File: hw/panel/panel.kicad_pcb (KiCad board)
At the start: 4 copper layers, 158 x 89 mm, 296 parts, among them J1 Input, J1 USB_OTG, J2 BATT, J2 Output, J201 Modem, J202 SIM_Card, J203 Motor, J204 Micro_SD_Card, J205 Prog, J206 Expansion, J207 Camera, J3 +5V, J301 iMX8, J305 Micro_SD_Card, J4 SJ-3571N, J401 Touch, J402 Display, J5 SPEAKER, SW1 RESET, SW2 WAKE, SW201 BOOT, SW202 PERST, U1 BQ25895, U1 SN65LVDS822, U10 74HC595, U11 ICS-43434, U12 MAX98357A, U13 MAX98357A, U14 SN74LVC1G04DCK, U15 SN74LVC1G3157DCK, U16 SN74LVC2G07DCK, U2 SN74LVC00ARGY, U2 TPS62293, U201 ESP32-WROOM, U202 SN74CBTLV3125RGY, U203 TXB0104RGY, U204 TXB0104RGY, U205 DRV2605LDGS, U206 LSM9DS1, U207 FT230XQ, U208 TMUX154ERSW, U3 TPS630250, U4 FE310-G002, U401 FAN5333BSX, U402 SN74LVC3G06DCU, U403 BT817Q, U404 IS25LP128-JKLE, U405 DS90C185, U406 TS3DV520ERUA, U407 TXS0104ERGY, U408 TXS0104ERGY, U409 SN74LVC2G06DCK, U5 IS25LP128-JKLE, U6 TMUX1574RSV, U7 74HC00, U8 74HC00, U9 74HC595, X1 SiT1533, Y1 16MHz, Y401 12MHz

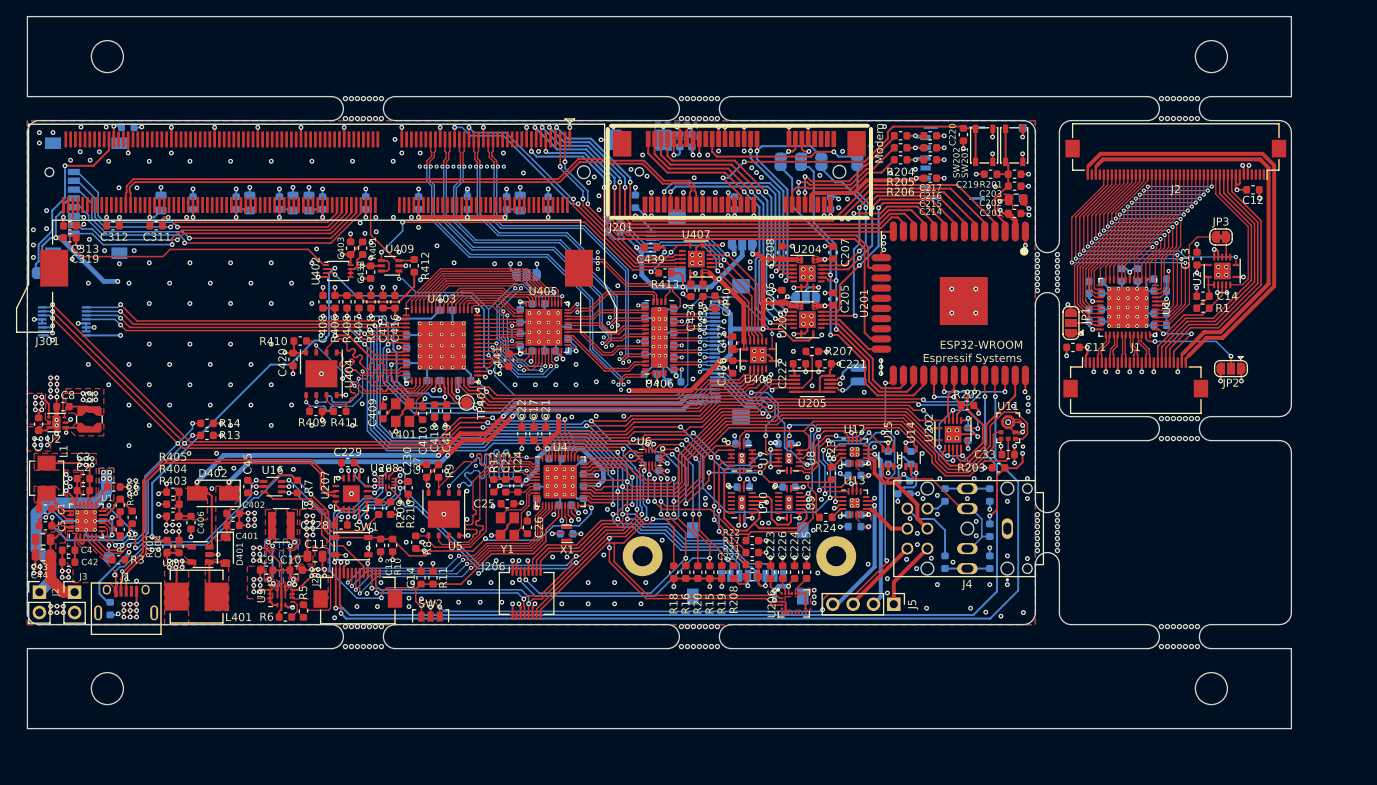
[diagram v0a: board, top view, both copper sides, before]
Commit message: temp commit for merge
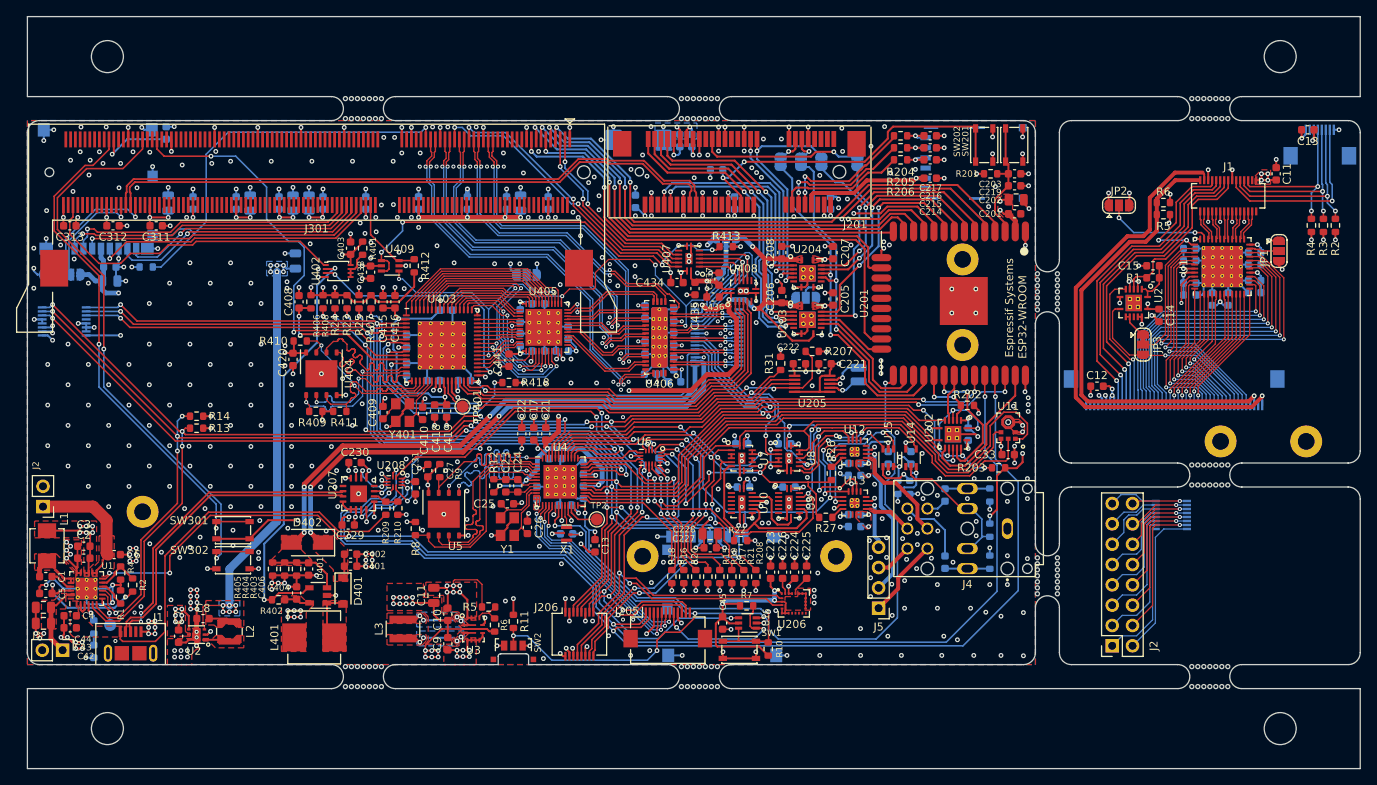
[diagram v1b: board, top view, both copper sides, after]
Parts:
- removed the C1 at (189.5, 86.6)
- removed the C1 at (58.2, 111.5)
- removed the C11 at (186.7, 91.3)
- removed the C11 at (92.0, 117.5)
- removed C439, C440: 0.1uF, Capacitor_SMD:C_0603_1608Metric
- removed the J1 at (194.6, 95.1)
- removed the J1 at (68.3, 123.4)
- removed the J2 at (199.6, 67.9)
- removed the J2 at (57.5, 122.0)
- removed the J3 at (61.9, 122.0)
- removed J305: Micro_SD_Card, footprints:microSD
- removed the R2 at (69.1, 112.6)
- removed the R3 at (67.4, 117.9)
- removed the R4 at (67.6, 111.1)
- removed R414, R415: R, Resistor_SMD:R_0603_1608Metric
- removed the R5 at (90.5, 124.3)
- removed the R6 at (88.2, 125.0)
- removed the REF** at (183.5, 114.5)
- removed the REF** at (183.5, 82.0)
- removed the REF** at (98.0, 127.5)
- removed the REF** at (140.0, 127.5)
- removed the REF** at (200.0, 127.5)
- removed the REF** at (200.0, 101.5)
- removed the REF** at (200.0, 61.5)
- removed the U2 at (205.3, 81.8)
- removed the U2 at (59.6, 100.8)
- added C1: 47nF, Capacitor_SMD:C_0603_1608Metric, F.Cu at (58.3, 120.0)
- added C1: 0.1uF, Capacitor_SMD:C_0603_1608Metric, B.Cu at (209.4, 81.0)
- added C11: 47uF, Capacitor_SMD:C_0805_2012Metric, F.Cu at (106.8, 122.3)
- added C11: 10uF, Capacitor_SMD:C_0603_1608Metric, F.Cu at (212.1, 69.7)
- added C13: 0.1uF, Capacitor_SMD:C_0603_1608Metric, F.Cu at (216.1, 64.2)
- added C228: 22uF, Capacitor_SMD:C_0805_2012Metric, F.Cu at (141.3, 114.7)
- added C320: 22uF, Capacitor_SMD:C_0805_2012Metric, B.Cu at (66.3, 83.0)
- added J1: USB_OTG, footprints:GCT_MicroUSB-USB3080, F.Cu at (68.9, 126.9)
- added J1: Input, Connector_Molex:Molex_SlimStack_55560-0301_2x15_P0.50mm_Vertical, F.Cu at (206.1, 72.4)
- added J1: In, Connector_Molex:Molex_SlimStack_55560-0161_2x08_P0.50mm_Vertical, B.Cu at (199.0, 112.3)
- added J2: BATT, Connector_PinHeader_2.54mm:PinHeader_1x02_P2.54mm_Vertical, F.Cu at (58.0, 111.2)
- added J2: Display, Connector_FFC-FPC:Hirose_FH12-45S-0.5SH_1x45-1MP_P0.50mm_Horizontal, B.Cu at (199.3, 96.7)
- added J2: Out, Connector_PinHeader_2.54mm:PinHeader_2x08_P2.54mm_Vertical, F.Cu at (191.6, 128.7)
- added J3: +5V, Connector_PinHeader_2.54mm:PinHeader_1x02_P2.54mm_Vertical, F.Cu at (60.4, 129.2)
- added J3: Touch, Connector_FFC-FPC:Hirose_FH12-8S-0.5SH_1x08-1MP_P0.50mm_Horizontal, B.Cu at (217.6, 66.0)
- added J302: Micro_SD_Card_Det, footprints:Molex_MicroSD-5027740891, B.Cu at (70.8, 63.3)
- added J303: Spacer, footprints:Spacer, F.Cu at (70.4, 111.9)
- added J4: Spacer, footprints:Spacer, F.Cu at (215.8, 103.1)
- added J403: Spacer, footprints:Spacer, B.Cu at (172.9, 91.0)
- added J5: Spacer, footprints:Spacer, F.Cu at (205.2, 103.1)
- added JP302: USB_ID, Jumper:SolderJumper-2_P1.3mm_Open_RoundedPad1.0x1.5mm, B.Cu at (58.6, 82.2)
- added R2: 10K, Resistor_SMD:R_0603_1608Metric, F.Cu at (69.2, 121.0)
- added R2: DNP, Resistor_SMD:R_0603_1608Metric, F.Cu at (219.5, 76.1)
- added R23: 100K, Resistor_SMD:R_0603_1608Metric, F.Cu at (96.0, 85.7)
- added R24: 100K, Resistor_SMD:R_0603_1608Metric, F.Cu at (94.5, 85.7)
- added R25: 100K, Resistor_SMD:R_0603_1608Metric, F.Cu at (97.5, 85.7)
- added R3: 2.2K, Resistor_SMD:R_0603_1608Metric, B.Cu at (64.3, 126.3)
- added R3: DNP, Resistor_SMD:R_0603_1608Metric, F.Cu at (218.0, 76.1)
- added R301: 100K, Resistor_SMD:R_0603_1608Metric, B.Cu at (70.8, 81.3)
- added R31: 100K, Resistor_SMD:R_0603_1608Metric, F.Cu at (150.2, 93.3)
- added R4: 10K, Resistor_SMD:R_0603_1608Metric, F.Cu at (67.7, 119.5)
- added R4: DNP, Resistor_SMD:R_0603_1608Metric, F.Cu at (216.5, 76.1)
- added R5: 560K, Resistor_SMD:R_0603_1608Metric, F.Cu at (113.7, 123.8)
- added R5: DNP, Resistor_SMD:R_0603_1608Metric, F.Cu at (198.0, 74.8)
- added R6: 180K, Resistor_SMD:R_0603_1608Metric, F.Cu at (114.4, 126.0)
- added R6: DNP, Resistor_SMD:R_0603_1608Metric, F.Cu at (198.0, 73.2)
- added REF**: mouse-bite-3mm-slot, panelization:mouse-bite-3mm-slot, F.Cu at (183.5, 119.9)
- added REF**: mouse-bite-3mm-slot, panelization:mouse-bite-3mm-slot, F.Cu at (183.5, 84.4)
- added REF**: mouse-bite-3mm-slot, panelization:mouse-bite-3mm-slot, F.Cu at (98.0, 132.5)
- added REF**: mouse-bite-3mm-slot, panelization:mouse-bite-3mm-slot, F.Cu at (140.0, 132.5)
- added REF**: mouse-bite-3mm-slot, panelization:mouse-bite-3mm-slot, F.Cu at (203.8, 132.5)
- added REF**: mouse-bite-3mm-slot, panelization:mouse-bite-3mm-slot, F.Cu at (203.8, 107.3)
- added REF**: mouse-bite-3mm-slot, panelization:mouse-bite-3mm-slot, F.Cu at (203.8, 61.5)
- added SW301: iMX8_ALT_BOOT, Button_Switch_SMD:SW_SPST_PTS810, F.Cu at (81.7, 114.2)
- added SW302: iMX8_RST, Button_Switch_SMD:SW_SPST_PTS810, F.Cu at (81.7, 118.0)
- added TP2: PMU_OUT0, TestPoint:TestPoint_Pad_D1.5mm, F.Cu at (127.2, 112.8)
- added U2: TPS62293, footprints:TPS62290, F.Cu at (77.2, 127.2)
- added U2: SN74LVC00ARGY, footprints:Texas_S-PVQFN-N14_ThermalVias, F.Cu at (194.3, 85.8)
- C14: value 10nF -> 22uF; footprint Capacitor_SMD:C_0603_1608Metric -> Capacitor_SMD:C_0805_2012Metric; moved to B.Cu
- C219: value 10nF -> 0.1uF
- C220: value 10nF -> 0.1uF; moved to B.Cu
- C319: moved to B.Cu
- J201: footprint footprints:Socket_mPCIe -> footprints:TE_mPCIe-1775862
- J204: value Micro_SD_Card -> Micro_SD_Card_Det; footprint footprints:microSD -> footprints:Molex_MicroSD-5027740891
- J301: footprint footprints:Socket_SODIMM_DDR3_TE_2013289 -> footprints:TE_SODIMMDDR3-2013289
- J401: value Touch -> Display; footprint Connector_FFC-FPC:Hirose_FH12-8S-0.5SH_1x08-1MP_P0.50mm_Horizontal -> Connector_Molex:Molex_SlimStack_54722-0304_2x15_P0.50mm_Vertical
- J402: value Display -> Spacer; footprint Connector_FFC-FPC:Hirose_FH12-26S-0.5SH_1x26-1MP_P0.50mm_Horizontal -> footprints:Spacer
- JP201: value LEVEL EN -> SIMCom_EN
- JP3: footprint Jumper:SolderJumper-2_P1.3mm_Bridged_RoundedPad1.0x1.5mm -> Jumper:SolderJumper-3_P1.3mm_Bridged12_RoundedPad1.0x1.5mm
- JP301: value ALT_BOOT -> USB_VBUS
- L2: footprint footprints:L_Coilcraft_LPS3015 -> footprints:Coilcraft-LPS3015
- L3: footprint footprints:L_Coilcraft_XAL40 -> footprints:Coilcraft-XAL40
- L401: footprint footprints:L_Murata_LQH66SN -> footprints:Murata-LQH66SN
- SW201: value BOOT -> ESP32_RST
- SW202: value PERST -> MODEM_RST
- U10, U9: footprint footprints:74HC595BQ115 -> footprints:DHVQFN-16_2.5x3.5mm_P0.5mm_EP1.0x2.0mm
- U202, U203, U204: footprint Package_DFN_QFN:Texas_S-PVQFN-N14_ThermalVias -> footprints:Texas_S-PVQFN-N14_ThermalVias
- U407, U408: footprint Package_DFN_QFN:Texas_S-PVQFN-N14_ThermalVias -> footprints:DHVQFN-14_2.5x3.0mm_P0.5mm_EP1.0x1.5mm
- U7, U8: footprint footprints:74HC00BQ115 -> footprints:DHVQFN-14_2.5x3.0mm_P0.5mm_EP1.0x1.5mm
- moved C45 61.8 mm to (142.9, 125.8)
- moved U16 61.8 mm to (146.0, 125.8)
- moved R7 58.1 mm to (145.9, 123.7), turned to 0 degrees
- moved SW1 50.2 mm to (145.0, 129.2)
- moved R10 48.7 mm to (148.6, 129.1)
- moved C14 42.6 mm to (89.5, 80.5)
- moved J205 39.1 mm to (136.1, 126.3)
- moved C7 31.8 mm to (74.9, 127.5)
- moved C8 31.8 mm to (78.0, 125.2)
- moved L2 31.8 mm to (81.2, 126.8)
- moved C12 31.4 mm to (189.7, 96.2), turned to 180 degrees
- moved J402 31.3 mm to (172.9, 80.3), turned to 0 degrees
- moved C220 31.2 mm to (142.2, 69.2), turned to 180 degrees
- moved JP1 27.5 mm to (212.4, 79.3), turned to 270 degrees
- moved C13 26.8 mm to (127.0, 116.2)
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- renumbered C13 to C14, C14 to C15, C228 to C229, C229 to C230, C230 to C231, R23 to R26, R24 to R27, R25 to R28, R26 to R29, R27 to R30, R28 to R32, R29 to R33
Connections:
- net Net-(TP401-Pad1) renamed /disp/BT81X_AUDIO
- net Net-(U4-Pad17) renamed /AON_PMU_OUT_1
- C14 pad 1: WAKE -> +1V8
- J204 pad 2: SPI1.SS3 -> GPIO_0
- J204 pad 9: GND -> Net-(J204-Pad9)
- J206 pad 10: UART0.TXD -> TMUX.I2C0.SCL
- J206 pad 11: SPI1.MOSI -> GND
- J206 pad 13: SPI1.MISO -> UART0.TXD
- J206 pad 14: TMUX.I2C0.SDA -> TMUX.GPIO1
- J206 pad 15: SPI1.SCK -> UART0.RXD
- J206 pad 16: TMUX.I2C0.SCL -> TMUX.GPIO0
- J206 pad 5: TMUX.GPIO0 -> SPI1.MOSI
- J206 pad 7: TMUX.GPIO1 -> SPI1.MISO
- J206 pad 8: UART0.RXD -> TMUX.I2C0.SDA
- J206 pad 9: GND -> SPI1.SCK
- J207 pad 1: GPIO_23 -> TMUX.I2C0.SCL
- J207 pad 3: TMUX.I2C0.SCL -> TMUX.I2C0.SDA
- J207 pad 5: TMUX.I2C0.SDA -> SPI1.SS2
- J207 pad 8: BT81X.GPIO0 -> Net-(J207-Pad8)
- J301 pad 165: Net-(J301-Pad165) -> BT81X.GPIO0
- J301 pad 171: Net-(J301-Pad171) -> /exp/RESET
- J301 pad 174: Net-(J301-Pad174) -> iMX8.USB1.ID
- J301 pad 180: Net-(J301-Pad180) -> iMX8.USB1.VBUS
- J301 pad 61: GND -> /exp/SD2_DET
- J401 pad 1: GND -> +3V3
- J401 pad 3: +VCTP -> +1V8
- J401 pad 4: /disp/CTP_SCL -> /disp/DISP_LVDS_A0N
- J401 pad 5: /disp/CTP_SDA -> /disp/CTP_SCL
- J401 pad 6: /disp/CTP_INT -> /disp/DISP_LVDS_A0P
- J401 pad 7: /disp/CTP_RST -> /disp/CTP_SDA
- J402 pad 1: +3V3 -> GND
- JP3 pad 1: /DISP_EN_IC -> Net-(JP3-Pad1)
- JP3 pad 2: Net-(JP3-Pad2) -> /DISP_DE_INV
- JP301 pad 1: /exp/ALT_BOOT -> +3V3
- JP301 pad 2: +3V3 -> iMX8.USB1.VBUS
- R208 pad 2: SPI1.SS3 -> GPIO_0
- R407 pad 2: SPI1.SS2 -> SPI1.SS3
- R408 pad 2: GPIO_0 -> GPIO_23
- SW2 pad 1: WAKE -> GND
- SW2 pad 2: GND -> WAKE
- U1 pad 38: /DISP_EN_IC -> /DISP_DE_INV
- U4 pad 22: Net-(U4-Pad22) -> /AON_PMU_OUT_0
- U403 pad 11: GPIO_0 -> GPIO_23
- U403 pad 6: SPI1.SS2 -> SPI1.SS3
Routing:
- net /exp/RESET: track 0.00 -> 73.1 mm, vias 0 -> 2
- net /BQ_QON: track 28.3 -> 93.0 mm
- net GND: track 570.8 -> 633.6 mm, vias 598 -> 674
- net +1V8: track 127.8 -> 186.8 mm, vias 23 -> 30
- net /exp/SD2_DET: track 0.00 -> 53.6 mm, vias 0 -> 1
- net /exp/ALT_BOOT: track 22.8 -> 65.4 mm, vias 1 -> 2
- net GPIO_0: track 63.7 -> 30.9 mm, vias 3 -> 2
- net SPI1.SS2: track 58.5 -> 88.5 mm
- net +VCTP: track 46.4 -> 16.5 mm, vias 3 -> 2
- net WAKE: track 143.7 -> 117.8 mm
- net CTP.INT: track 0.00 -> 23.8 mm, vias 0 -> 2
- net GPIO_23: track 79.6 -> 55.9 mm, vias 3 -> 5
- net SPI1.SS3: track 33.5 -> 56.9 mm, vias 4 -> 3
- net CTP.RST: track 0.00 -> 22.6 mm, vias 0 -> 1
- net CTP.SDA: track 0.00 -> 22.0 mm, vias 0 -> 2
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- removed copper zone on F.Cu, net +VCTP
- removed copper zone on B.Cu, net DISP_LED_A
- removed copper zone on B.Cu, net Net-(C6-Pad1)
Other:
- board size 158 x 89 mm -> 166.6 x 94 mm
- net class AUDIO removed
- net class BT81X removed
- net class CTP removed
- net class DISPLAY removed
- net class Default: clearance 0.2 -> 0.1524; trace_width 0.25 -> 0.1524; via_dia 0.6 -> 0.508; via_drill 0.3 -> 0.254
- net class FE310 removed
- net class FE310_L removed
- net class USB removed
- net class USB2DIFF removed
- rule pad_to_mask_clearance: 0.05 -> 0
- rule trace_clearance: 0.2 -> 0.1524
- rule via_min_size: 0.5 -> 0.4
